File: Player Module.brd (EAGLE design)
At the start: 76.2 x 101.6 mm, 25 parts, among them U3 5V, U4 STM32F0XXC1T, U5 PCF8574T/3,512SOT162-1-M, U7 3.3V/150mA

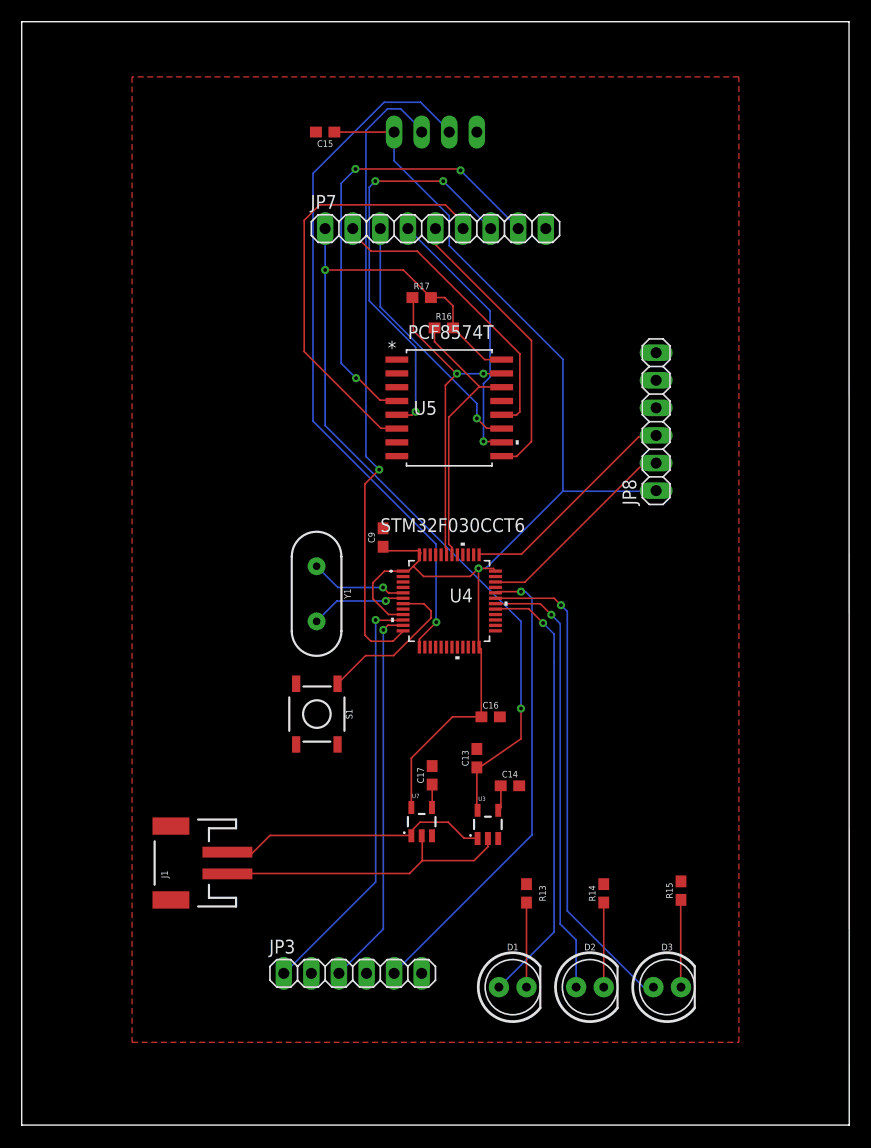
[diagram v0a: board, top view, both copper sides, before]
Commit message: updates as of wednesday night
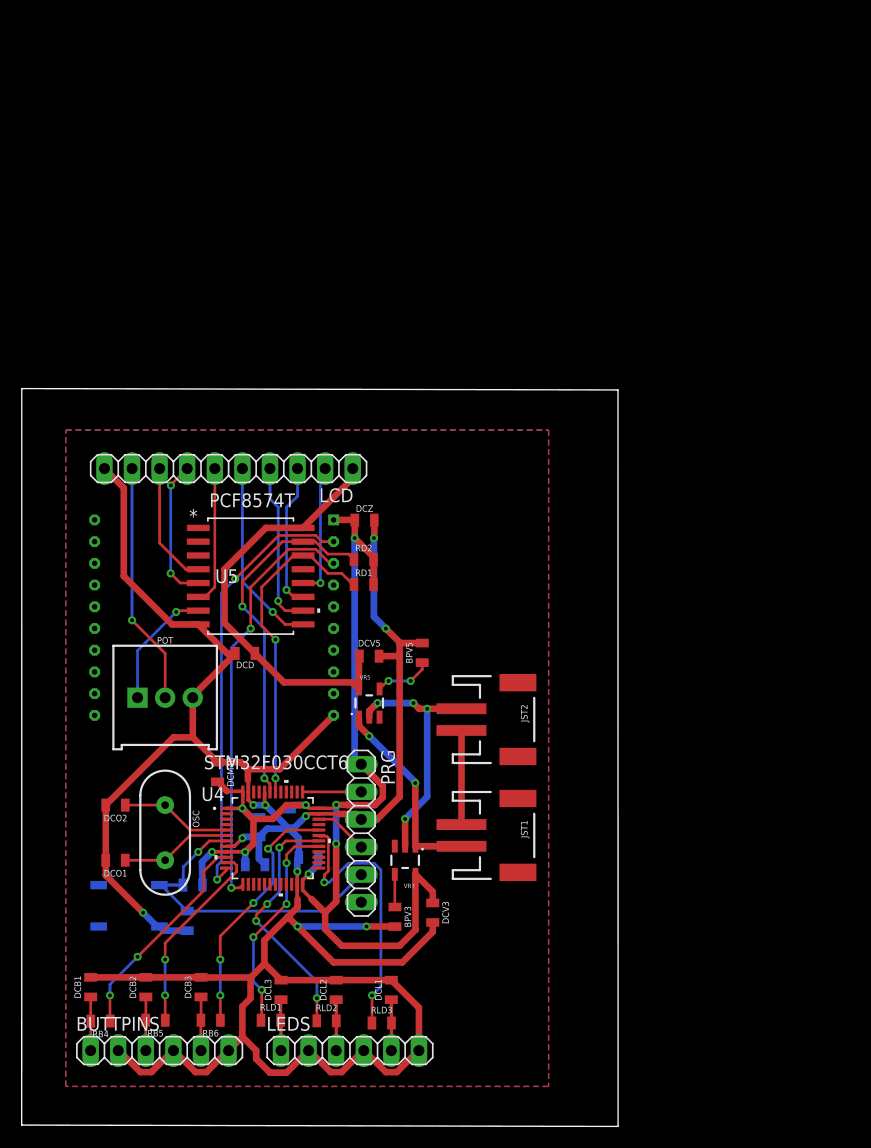
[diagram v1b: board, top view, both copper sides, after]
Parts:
- removed C13, C15, C16: 2.2uF, SparkFun-Capacitors:0603
- removed C14, C17: 470pF, SparkFun-Capacitors:0603
- removed C9: 10uF, SparkFun-Capacitors:0603
- removed D1, D2, D3: (no value), SparkFun-LED:LED_5MM
- removed J1: (no value), SparkFun-Connectors:JST-2-SMD
- removed JP3, JP8: (no value), pinhead:1X06
- removed JP5: (no value), pinhead:1X04
- removed JP7: (no value), pinhead:1X09
- removed R13, R14, R15, R16, R17: (no value), SparkFun-Resistors:0603
- removed U3: 5V, SparkFun-IC-Power:SOT23-5
- removed U7: 3.3V/150mA, SparkFun-IC-Power:SOT23-5
- removed Y1: (no value), SparkFun-Clocks:HC49US
- added BPV3, BPV5: 470pF, SparkFun-Capacitors:0805
- added BUTTPINS, LEDS, PRG: (no value), pinhead:1X06
- added DCB1, DCB2, DCB3, DCD, DCL1, DCL2, DCL3, DCM1, DCM24, DCM36, DCM48, DCM9, DCO1, DCO2, DCSW, DCZ: 0.33µF, SparkFun-Capacitors:0805
- added DCV3, DCV5: 2.2µF, SparkFun-Capacitors:0805
- added JST1, JST2: (no value), SparkFun-Connectors:JST-2-SMD
- added LCD: (no value), pinhead:1X10
- added OSC: (no value), SparkFun-Clocks:HC49US
- added POT: 10k, SparkFun-Resistors:TRIMPOT-PTH-3386U
- added RB4, RB5, RB6, RLD1, RLD2, RLD3: 1k, SparkFun-Resistors:0805
- added RD1, RD2: 4.7k, SparkFun-Resistors:0805
- added RSW: 10k, SparkFun-Resistors:0805
- added U$1: XB24-BPIT-004, XB24-BPIT-004:DIP-20
- added VR3: 3.3V/150mA, SparkFun-IC-Power:SOT23-5
- added VR5: 5V, SparkFun-IC-Power:SOT23-5
- moved U4 27.2 mm to (23.1, 26.4)
- moved S1 24.7 mm to (9.88, 20.2), flipped to the bottom, turned to 0 degrees
- moved U5 24.0 mm to (21.1, 50.5)
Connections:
- removed net A13: JP8.2, U4.34
- removed net A14: JP8.3, U4.37
- removed net D0: JP7.8, U5.4
- removed net D1: JP7.7, U5.5
- removed net D2: JP7.6, U5.6
- removed net D4: JP7.5, U5.9
- removed net D5: JP7.4, U5.10
- removed net D6: JP7.3, U5.11
- removed net D7: JP7.2, U5.12
- removed net N$32: J1.1, U3.2, U7.2
- removed net N$38: J1.2, U3.1, U7.1
- removed net N$39: D1.K, R13.1
- removed net N$41: D2.K, R14.1
- removed net N$42: D3.K, R15.1
- new net GND_IN: JST2.1, VR3.2, VR5.2
- new net N$1: JST1.1, JST2.2
- new net N$11: LCD.4, U5.10
- new net N$12: LCD.5, U5.9
- new net N$13: BUTTPINS.3, DCB2.1, RB5.2
- new net N$14: LCD.6, U5.6
- new net N$15: LCD.7, U5.5
- new net N$16: LCD.8, U5.4
- new net N$17: BUTTPINS.5, DCB3.1, RB6.2
- new net N$3: DCL3.1, LEDS.1, RLD1.2
- new net N$4: DCL2.1, LEDS.3, RLD2.2
- new net N$5: DCL1.1, LEDS.5, RLD3.2
- new net N$8: BUTTPINS.1, DCB1.1, RB4.2
- new net N$9: LCD.2, U5.12
- new net POT_A: POT.1, U5.7
- new net POT_B: LCD.9, POT.2
- new net PWR_IN: JST1.2, VR3.1, VR5.1
- new net RST: DCSW.1, PRG.5, RSW.2, S1.1, U4.7
- new net SWCLK: PRG.2, U4.37
- new net SWDIO: PRG.4, U4.34
- net A0: now also RB4.1; no longer JP3.1
- net A1: now also RB5.1; no longer JP3.3
- net A10: now also RLD3.1; no longer D3.A
- net A11: now also RB6.1; no longer JP3.5
- net A2: now also U$1.2; no longer JP5.2
- net A3: now also U$1.3; no longer JP5.3
- net A8: now also RLD1.1; no longer D1.A
- net A9: now also RLD2.1; no longer D2.A
- net B6: now also RD1.1; no longer R16.1
- net B7: now also RD2.1; no longer R17.1
- net GND: now also BPV3.2, BPV5.2, BUTTPINS.2, BUTTPINS.4, BUTTPINS.6, DCB1.2, DCB2.2, DCB3.2, DCD.2, DCL1.2, DCL2.2, DCL3.2, DCM1.1, DCM24.1, DCM36.1, DCM48.1, DCM9.1, DCO1.2, DCO2.2, DCSW.2, DCV3.2, DCV5.2, DCZ.2, LCD.10, LEDS.2, LEDS.4, LEDS.6, POT.3, PRG.3, U$1.10; no longer C13.2, C14.2, C15.2, C16.2, C17.2, C9.2, JP3.2, JP3.4, JP3.6, JP5.4, JP7.9, JP8.6, R13.2, R14.2, R15.2
- net N$10: now also LCD.3, U5.11; no longer S1.1, U4.7
- net N$21: now also DCO2.1, OSC.1; no longer Y1.1
- net N$22: now also DCO1.1, OSC.2; no longer Y1.2
- net N$34: now also BPV3.1, VR3.4; no longer C17.1, U7.4
- net N$37: now also BPV5.1, VR5.4; no longer C14.1, U3.4
- net P3.3V: now also DCM1.2, DCM24.2, DCM36.2, DCM48.2, DCM9.2, DCV3.1, DCZ.1, PRG.1, RD1.2, RD2.2, RSW.1, U$1.1, VR3.5; no longer C15.1, C16.1, C9.1, JP5.1, JP8.1, U7.5
- net P5V: now also DCD.1, DCV5.1, LCD.1, VR5.5; no longer C13.1, JP7.1, R16.2, R17.2, U3.5
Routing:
- net GND: track 0.00 -> 256.4 mm, vias 0 -> 10
- net P5V: track 84.2 -> 39.0 mm, vias 2 -> 0
- net D0: track 42.5 -> 0.00 mm, vias 3 -> 0
- net D2: track 40.0 -> 0.00 mm
- net D1: track 37.5 -> 0.00 mm, vias 3 -> 0
- net RST: track 0.00 -> 29.6 mm, vias 0 -> 1
- net N$32: track 28.1 -> 0.00 mm
- net D7: track 27.6 -> 0.00 mm
- net D4: track 26.6 -> 0.00 mm
- net A3: track 65.6 -> 39.2 mm, vias 1 -> 2
- net N$38: track 25.2 -> 0.00 mm
- net D5: track 24.7 -> 0.00 mm, vias 1 -> 0
- net D6: track 23.8 -> 0.00 mm, vias 1 -> 0
- net GND_IN: track 0.00 -> 23.1 mm, vias 0 -> 4
- net POT_B: track 0.00 -> 22.4 mm, vias 0 -> 1
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- added copper zone on layer 16, net GND
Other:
- board size 76.2 x 101.6 mm -> 54.9 x 67.9 mm

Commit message: final stuff
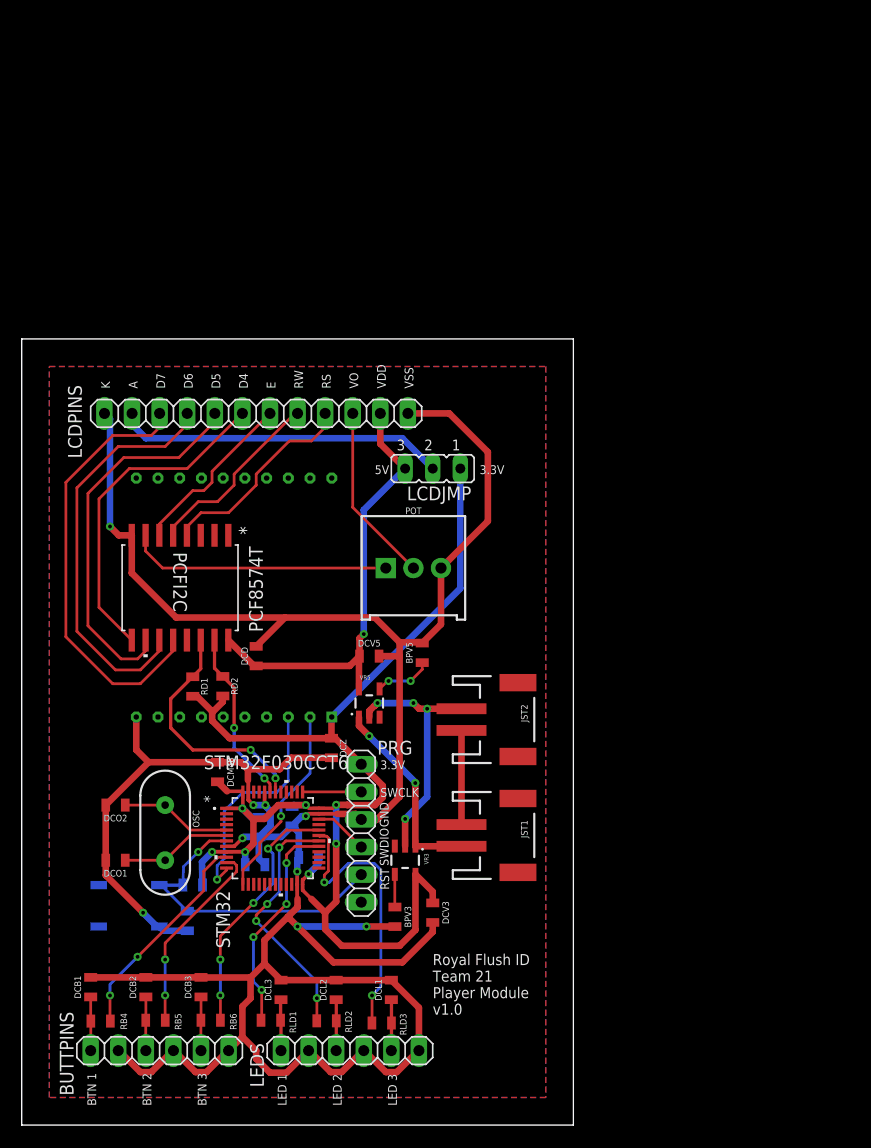
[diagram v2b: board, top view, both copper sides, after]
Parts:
- removed LCD: (no value), pinhead:1X10
- removed U$1: XB24-BPIT-004, XB24-BPIT-004:DIP-20
- removed U5: PCF8574T/3,512SOT162-1-M, ECE477_Resources:SOT162-1-M
- added LCDJMP: (no value), jumper:JP2
- added LCDPINS: (no value), pinhead:1X12
- added PCFI2C: PCF8574T/3,512SOT162-1-M, ECE477_Resources:SOT162-1-M
- added XBEE: XB24-BPIT-004, XB24-BPIT-004:DIP-20
- moved POT 25.8 mm to (36.1, 51.3)
- moved DCZ 21.2 mm to (28.5, 34.7), turned to 270 degrees
- moved RD1 18.3 mm to (15.7, 40.4), turned to 270 degrees
- moved RD2 17.4 mm to (18.5, 40.4), turned to 270 degrees
- moved DCD 1.05 mm to (21.6, 43.2), turned to 90 degrees
- moved DCM36 0.36 mm to (24.9, 28.4)
- renumbered U4 to STM32
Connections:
- net A0 renamed PA0
- net A1 renamed PA1
- net A10 renamed PA10
- net A11 renamed PA11
- net A8 renamed PA8
- net A9 renamed PA9
- removed net A2: STM32.12, U$1.2
- removed net A3: STM32.13, U$1.3
- removed net A4: STM32.14
- removed net A5: STM32.15
- removed net A6: STM32.16
- removed net A7: STM32.17
- removed net B6: RD1.1, STM32.42, U5.14
- removed net B7: RD2.1, STM32.43, U5.15
- removed net N$10: LCD.3, U5.11
- removed net N$11: LCD.4, U5.10
- removed net N$12: LCD.5, U5.9
- removed net N$14: LCD.6, U5.6
- removed net N$15: LCD.7, U5.5
- removed net N$16: LCD.8, U5.4
- removed net N$9: LCD.2, U5.12
- new net A: LCDJMP.2, LCDPINS.2
- new net D4: LCDPINS.6, PCFI2C.9
- new net D5: LCDPINS.5, PCFI2C.10
- new net D6: LCDPINS.4, PCFI2C.11
- new net D7: LCDPINS.3, PCFI2C.12
- new net E: LCDPINS.7, PCFI2C.6
- new net RS: LCDPINS.9, PCFI2C.4
- new net RW: LCDPINS.8, PCFI2C.5
- new net RX: STM32.12, XBEE.3
- new net SCL: PCFI2C.14, RD1.1, STM32.42
- new net SDA: PCFI2C.15, RD2.1, STM32.43
- new net TX: STM32.13, XBEE.2
- net GND: now also LCDPINS.1, LCDPINS.12, PCFI2C.8, XBEE.10; no longer LCD.10, U$1.10, U5.8
- net P3.3V: now also LCDJMP.1, XBEE.1; no longer U$1.1
- net P5V: now also LCDJMP.3, LCDPINS.11, PCFI2C.16; no longer LCD.1, U5.16
- net POT_A: now also PCFI2C.7; no longer U5.7
- net POT_B: now also LCDPINS.10; no longer LCD.9
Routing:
- net A2: track 40.7 -> 0.00 mm, vias 2 -> 0
- net D7: track 0.00 -> 40.1 mm
- net A3: track 39.2 -> 0.00 mm, vias 2 -> 0
- net D6: track 0.00 -> 37.6 mm
- net D5: track 0.00 -> 35.2 mm
- net B7: track 32.9 -> 0.00 mm, vias 2 -> 0
- net GND: track 256.4 -> 288.9 mm, vias 10 -> 9
- net D4: track 0.00 -> 30.7 mm
- net A: track 0.00 -> 30.4 mm
- net B6: track 30.2 -> 0.00 mm, vias 2 -> 0
- net SCL: track 0.00 -> 22.3 mm, vias 0 -> 2
- net RX: track 0.00 -> 20.9 mm, vias 0 -> 1
- net P3.3V: track 104.7 -> 124.9 mm, vias 8 -> 7
- net RS: track 0.00 -> 19.2 mm
- net TX: track 0.00 -> 18.0 mm, vias 0 -> 1
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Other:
- board size 54.9 x 67.9 mm -> 50.8 x 72.4 mm
- board text added: "*"
- board text added: "3.3V"
- board text added: "5V"
- board text added: "A"
- board text added: "BTN 1"
- board text added: "BTN 2"
- board text added: "BTN 3"
- board text added: "D4"
- board text added: "D5"
- board text added: "D6"
- board text added: "D7"
- board text added: "E"
- board text added: "GND"
- board text added: "K"
- board text added: "LED 1"
- board text added: "LED 2"
- board text added: "LED 3"
- board text added: "RS"
- board text added: "RST"
- board text added: "RW"
- board text added: "RX"
- board text added: "Royal Flush ID Team 21 Player Module v1.0"
- board text added: "SWCLK"
- board text added: "SWDIO"
- board text added: "TX"
- board text added: "VDD"
- board text added: "VO"
- board text added: "VSS"
